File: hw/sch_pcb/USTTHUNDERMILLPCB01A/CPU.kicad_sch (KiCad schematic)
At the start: 28 parts, among them J4 HEADER_2x03, J5 SM08B-GHS-TB, J6 SM06B-GHS-TB, U7 SHT31, U8 ATMEGA1284P-AU, U9 AT24CS64-SSHM, Y1 16MHz

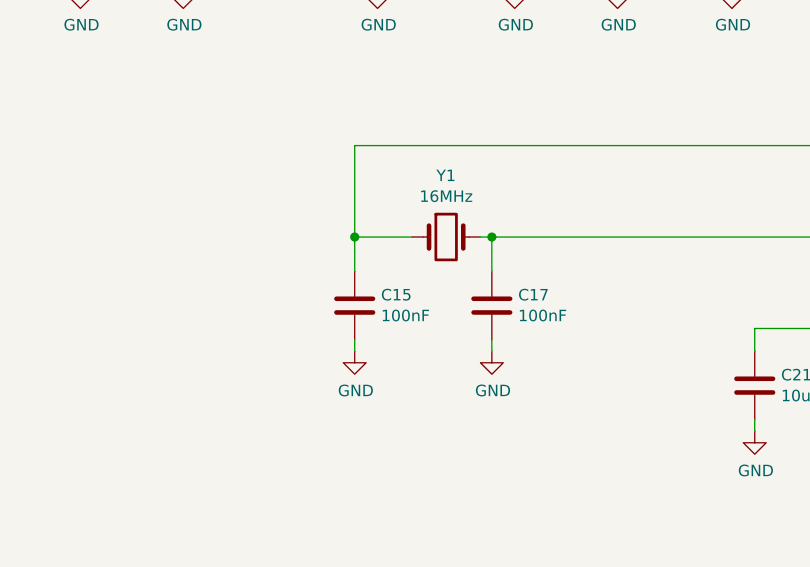
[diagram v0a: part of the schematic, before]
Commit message: Edit PCB
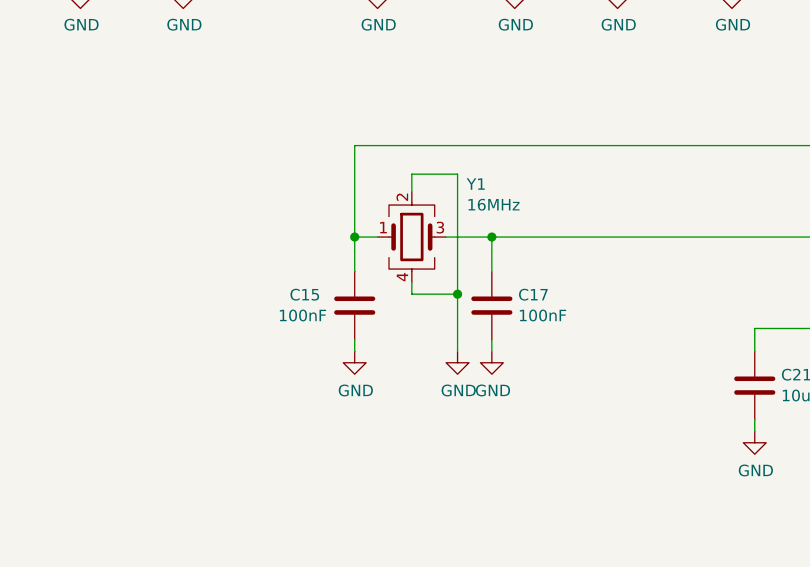
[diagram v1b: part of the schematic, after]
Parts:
- removed Y1: 16MHz, Mlab_XTAL:Crystal_HC49-U_Vertical, symbol Device:Crystal
- added Y1: 16MHz, Mlab_XTAL:Crystal SMD CFPX-180, symbol Device:Crystal_GND24
- J4: footprint Mlab_Pin_Headers:Straight_2x03 -> Mlab_Pin_Headers:SMD_2x03
- L1: footprint Mlab_R:SMD-1210 -> Inductor_SMD:L_1210_3225Metric
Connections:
- net GND: now also Y1.2, Y1.4
- net at C15.1, U8.7 (XTAL2): now also Y1.1
- net at C17.1, U8.8 (XTAL1): now also Y1.3
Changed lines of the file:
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@@
   (junction (at 62.23 20.955) (diameter 1.016) (color 0 0 0 0))
   (junction (at 64.77 168.275) (diameter 1.016) (color 0 0 0 0))
+  (junction (at 71.12 65.405) (diameter 1.016) (color 0 0 0 0))
   (junction (at 74.93 59.055) (diameter 1.016) (color 0 0 0 0))
   (junction (at 115.57 69.215) (diameter 1.016) (color 0 0 0 0))
@@
     (stroke (width 0) (type solid) (color 0 0 0 0))
   )
+  (wire (pts (xy 59.69 59.055) (xy 62.23 59.055))
+    (stroke (width 0) (type solid) (color 0 0 0 0))
+  )
   (wire (pts (xy 59.69 71.755) (xy 59.69 70.485))
     (stroke (width 0) (type solid) (color 0 0 0 0))
@@
     (stroke (width 0) (type solid) (color 0 0 0 0))
   )
-  (wire (pts (xy 66.04 59.055) (xy 59.69 59.055))
-    (stroke (width 0) (type solid) (color 0 0 0 0))
-  )
-  (wire (pts (xy 74.93 59.055) (xy 73.66 59.055))
+  (wire (pts (xy 66.04 52.07) (xy 66.04 53.975))
+    (stroke (width 0) (type solid) (color 0 0 0 0))
+  )
+  (wire (pts (xy 66.04 52.07) (xy 71.12 52.07))
+    (stroke (width 0) (type solid) (color 0 0 0 0))
+  )
+  (wire (pts (xy 66.04 64.135) (xy 66.04 65.405))
+    (stroke (width 0) (type solid) (color 0 0 0 0))
+  )
+  (wire (pts (xy 66.04 65.405) (xy 71.12 65.405))
+    (stroke (width 0) (type solid) (color 0 0 0 0))
+  )
+  (wire (pts (xy 69.85 59.055) (xy 74.93 59.055))
+    (stroke (width 0) (type solid) (color 0 0 0 0))
+  )
+  (wire (pts (xy 71.12 52.07) (xy 71.12 65.405))
+    (stroke (width 0) (type solid) (color 0 0 0 0))
+  )
+  (wire (pts (xy 71.12 65.405) (xy 71.12 71.755))
     (stroke (width 0) (type solid) (color 0 0 0 0))
   )
@@
     (pin "1")
   )
+  (symbol (lib_id "power:GND") (at 71.12 71.755 0) (unit 1)
+    (in_bom yes) (on_board yes)
+    (property "Reference" "#PWR0101" (id 0) (at 71.12 78.105 0)
+      (effects (font (size 1.27 1.27)) hide)
+    )
+    (property "Value" "GND" (id 1) (at 71.247 76.1492 0))
+    (property "Footprint" "" (id 2) (at 71.12 71.755 0)
+      (effects (font (size 1.27 1.27)) hide)
+    )
+    (property "Datasheet" "" (id 3) (at 71.12 71.755 0)
+      (effects (font (size 1.27 1.27)) hide)
+    )
+    (pin "1")
+  )
   (symbol (lib_id "power:GND") (at 74.93 71.755 0) (unit 1)
     (in_bom yes) (on_board yes)
@@
     (property "Reference" "L1" (id 0) (at 52.07 16.129 90))
     (property "Value" "10uH - LQH32CN100K23L" (id 1) (at 52.07 18.4404 90))
-    (property "Footprint" "Mlab_R:SMD-1210" (id 2) (at 52.07 20.955 0)
+    (property "Footprint" "Inductor_SMD:L_1210_3225Metric" (id 2) (at 52.07 20.955 0)
       (effects (font (size 1.27 1.27)) hide)
     )
@@
   (symbol (lib_id "DATALOGGER01A-rescue:C-device") (at 59.69 66.675 0) (unit 1)
     (in_bom yes) (on_board yes)
-    (property "Reference" "C15" (id 0) (at 62.611 65.5066 0)
-      (effects (font (size 1.27 1.27)) (justify left))
-    )
-    (property "Value" "100nF" (id 1) (at 62.611 67.818 0)
+    (property "Reference" "C15" (id 0) (at 52.451 65.5066 0)
+      (effects (font (size 1.27 1.27)) (justify left))
+    )
+    (property "Value" "100nF" (id 1) (at 51.181 67.818 0)
       (effects (font (size 1.27 1.27)) (justify left))
     )
@@
     (pin "2")
   )
-  (symbol (lib_id "Device:Crystal") (at 69.85 59.055 0) (unit 1)
-    (in_bom yes) (on_board yes)
-    (property "Reference" "Y1" (id 0) (at 69.85 52.2478 0))
-    (property "Value" "16MHz" (id 1) (at 69.85 54.5592 0))
-    (property "Footprint" "Mlab_XTAL:Crystal_HC49-U_Vertical" (id 2) (at 69.85 59.055 0)
-      (effects (font (size 1.27 1.27)) hide)
-    )
-    (property "Datasheet" "~" (id 3) (at 69.85 59.055 0)
-      (effects (font (size 1.27 1.27)) hide)
-    )
-    (property "USD_ID" "" (id 4) (at 69.85 59.055 0)
-      (effects (font (size 1.27 1.27)) hide)
-    )
-    (property "UST_ID" "" (id 5) (at 69.85 59.055 0)
-      (effects (font (size 1.27 1.27)) hide)
-    )
-    (pin "1")
-    (pin "2")
+  (symbol (lib_id "Device:Crystal_GND24") (at 66.04 59.055 0) (unit 1)
+    (in_bom yes) (on_board yes)
+    (property "Reference" "Y1" (id 0) (at 72.1361 53.2141 0)
+      (effects (font (size 1.27 1.27)) (justify left))
+    )
+    (property "Value" "16MHz" (id 1) (at 72.1361 55.5128 0)
+      (effects (font (size 1.27 1.27)) (justify left))
+    )
+    (property "Footprint" "Mlab_XTAL:Crystal SMD CFPX-180" (id 2) (at 66.04 59.055 0)
+      (effects (font (size 1.27 1.27)) hide)
+    )
+    (property "Datasheet" "LFXTAL035264REEL" (id 3) (at 66.04 59.055 0)
+      (effects (font (size 1.27 1.27)) hide)
+    )
+    (pin "1")
+    (pin "2")
+    (pin "3")
+    (pin "4")
   )
   (symbol (lib_id "DATALOGGER01A-rescue:HEADER_2x03-MLAB_HEADER") (at 148.59 158.115 0) (unit 1)
@@
       (effects (font (size 1.524 1.524)) hide)
     )
-    (property "Footprint" "Mlab_Pin_Headers:Straight_2x03" (id 2) (at 148.59 155.575 0)
+    (property "Footprint" "Mlab_Pin_Headers:SMD_2x03" (id 2) (at 148.59 155.575 0)
       (effects (font (size 1.524 1.524)) hide)
     )
